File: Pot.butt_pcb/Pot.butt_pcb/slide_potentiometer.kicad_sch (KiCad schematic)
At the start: 16 parts

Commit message: main_func pcb done
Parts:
- RV13, RV14, RV15, RV16, RV17, RV18, RV19, RV20: footprint (none) -> Connector_PinSocket_2.54mm:PinSocket_1x03_P2.54mm_Horizontal
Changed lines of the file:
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@@
       (effects (font (size 1.27 1.27)) (justify right))
     )
-    (property "Footprint" "" (id 2) (at 243.84 46.99 0)
+    (property "Footprint" "Connector_PinSocket_2.54mm:PinSocket_1x03_P2.54mm_Horizontal" (id 2) (at 243.84 46.99 0)
       (effects (font (size 1.27 1.27)) hide)
     )
@@
       (effects (font (size 1.27 1.27)) (justify right))
     )
-    (property "Footprint" "" (id 2) (at 179.07 48.26 0)
+    (property "Footprint" "Connector_PinSocket_2.54mm:PinSocket_1x03_P2.54mm_Horizontal" (id 2) (at 179.07 48.26 0)
       (effects (font (size 1.27 1.27)) hide)
     )
@@
       (effects (font (size 1.27 1.27)) (justify right))
     )
-    (property "Footprint" "" (id 2) (at 52.07 44.45 0)
+    (property "Footprint" "Connector_PinSocket_2.54mm:PinSocket_1x03_P2.54mm_Horizontal" (id 2) (at 52.07 44.45 0)
       (effects (font (size 1.27 1.27)) hide)
     )
@@
       (effects (font (size 1.27 1.27)) (justify right))
     )
-    (property "Footprint" "" (id 2) (at 242.57 93.98 0)
+    (property "Footprint" "Connector_PinSocket_2.54mm:PinSocket_1x03_P2.54mm_Horizontal" (id 2) (at 242.57 93.98 0)
       (effects (font (size 1.27 1.27)) hide)
     )
@@
       (effects (font (size 1.27 1.27)) (justify right))
     )
-    (property "Footprint" "" (id 2) (at 179.07 93.98 0)
+    (property "Footprint" "Connector_PinSocket_2.54mm:PinSocket_1x03_P2.54mm_Horizontal" (id 2) (at 179.07 93.98 0)
       (effects (font (size 1.27 1.27)) hide)
     )
@@
       (effects (font (size 1.27 1.27)) (justify right))
     )
-    (property "Footprint" "" (id 2) (at 115.57 45.72 0)
+    (property "Footprint" "Connector_PinSocket_2.54mm:PinSocket_1x03_P2.54mm_Horizontal" (id 2) (at 115.57 45.72 0)
       (effects (font (size 1.27 1.27)) hide)
     )
@@
       (effects (font (size 1.27 1.27)) (justify right))
     )
-    (property "Footprint" "" (id 2) (at 115.57 93.98 0)
+    (property "Footprint" "Connector_PinSocket_2.54mm:PinSocket_1x03_P2.54mm_Horizontal" (id 2) (at 115.57 93.98 0)
       (effects (font (size 1.27 1.27)) hide)
     )
@@
       (effects (font (size 1.27 1.27)) (justify right))
     )
-    (property "Footprint" "" (id 2) (at 52.07 93.98 0)
-      (effects (font (size 1.27 1.27)) hide)
-    )
+    (property "Footprint" "Connector_PinSocket_2.54mm:PinSocket_1x03_P2.54mm_Horizontal" (id 2) (at 52.07 93.98 0)
+      (effects (font (size 1.27 1.27)) hide)
+    )

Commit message: Pot.but_pcb in progress
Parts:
- RV13, RV14, RV15, RV16, RV17, RV18, RV19, RV20: footprint Connector_PinSocket_2.54mm:PinSocket_1x03_P2.54mm_Horizontal -> Connector_PinSocket_2.54mm:PinSocket_1x03_P2.54mm_Vertical
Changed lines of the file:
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@@
       (effects (font (size 1.27 1.27)) (justify right))
     )
-    (property "Footprint" "Connector_PinSocket_2.54mm:PinSocket_1x03_P2.54mm_Horizontal" (id 2) (at 243.84 46.99 0)
+    (property "Footprint" "Connector_PinSocket_2.54mm:PinSocket_1x03_P2.54mm_Vertical" (id 2) (at 243.84 46.99 0)
       (effects (font (size 1.27 1.27)) hide)
     )
@@
       (effects (font (size 1.27 1.27)) (justify right))
     )
-    (property "Footprint" "Connector_PinSocket_2.54mm:PinSocket_1x03_P2.54mm_Horizontal" (id 2) (at 179.07 48.26 0)
+    (property "Footprint" "Connector_PinSocket_2.54mm:PinSocket_1x03_P2.54mm_Vertical" (id 2) (at 179.07 48.26 0)
       (effects (font (size 1.27 1.27)) hide)
     )
@@
       (effects (font (size 1.27 1.27)) (justify right))
     )
-    (property "Footprint" "Connector_PinSocket_2.54mm:PinSocket_1x03_P2.54mm_Horizontal" (id 2) (at 52.07 44.45 0)
+    (property "Footprint" "Connector_PinSocket_2.54mm:PinSocket_1x03_P2.54mm_Vertical" (id 2) (at 52.07 44.45 0)
       (effects (font (size 1.27 1.27)) hide)
     )
@@
       (effects (font (size 1.27 1.27)) (justify right))
     )
-    (property "Footprint" "Connector_PinSocket_2.54mm:PinSocket_1x03_P2.54mm_Horizontal" (id 2) (at 242.57 93.98 0)
+    (property "Footprint" "Connector_PinSocket_2.54mm:PinSocket_1x03_P2.54mm_Vertical" (id 2) (at 242.57 93.98 0)
       (effects (font (size 1.27 1.27)) hide)
     )
@@
       (effects (font (size 1.27 1.27)) (justify right))
     )
-    (property "Footprint" "Connector_PinSocket_2.54mm:PinSocket_1x03_P2.54mm_Horizontal" (id 2) (at 179.07 93.98 0)
+    (property "Footprint" "Connector_PinSocket_2.54mm:PinSocket_1x03_P2.54mm_Vertical" (id 2) (at 179.07 93.98 0)
       (effects (font (size 1.27 1.27)) hide)
     )
@@
       (effects (font (size 1.27 1.27)) (justify right))
     )
-    (property "Footprint" "Connector_PinSocket_2.54mm:PinSocket_1x03_P2.54mm_Horizontal" (id 2) (at 115.57 45.72 0)
+    (property "Footprint" "Connector_PinSocket_2.54mm:PinSocket_1x03_P2.54mm_Vertical" (id 2) (at 115.57 45.72 0)
       (effects (font (size 1.27 1.27)) hide)
     )
@@
       (effects (font (size 1.27 1.27)) (justify right))
     )
-    (property "Footprint" "Connector_PinSocket_2.54mm:PinSocket_1x03_P2.54mm_Horizontal" (id 2) (at 115.57 93.98 0)
+    (property "Footprint" "Connector_PinSocket_2.54mm:PinSocket_1x03_P2.54mm_Vertical" (id 2) (at 115.57 93.98 0)
       (effects (font (size 1.27 1.27)) hide)
     )
@@
       (effects (font (size 1.27 1.27)) (justify right))
     )
-    (property "Footprint" "Connector_PinSocket_2.54mm:PinSocket_1x03_P2.54mm_Horizontal" (id 2) (at 52.07 93.98 0)
-      (effects (font (size 1.27 1.27)) hide)
-    )
+    (property "Footprint" "Connector_PinSocket_2.54mm:PinSocket_1x03_P2.54mm_Vertical" (id 2) (at 52.07 93.98 0)
+      (effects (font (size 1.27 1.27)) hide)
+    )

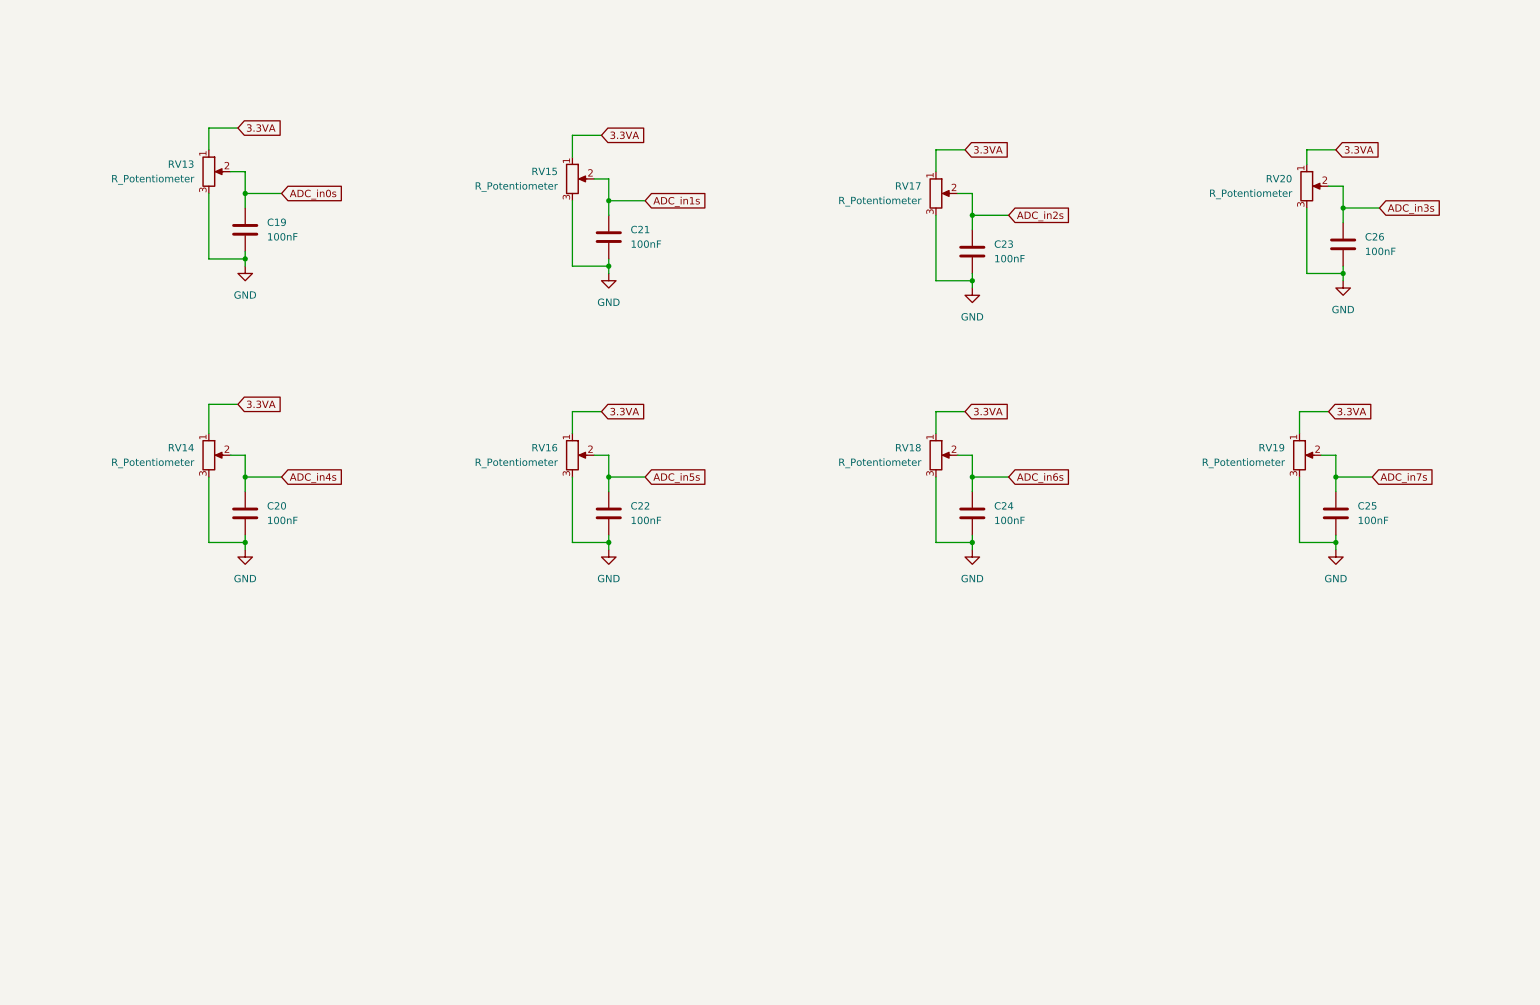
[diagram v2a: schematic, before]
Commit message: pcb design fixing
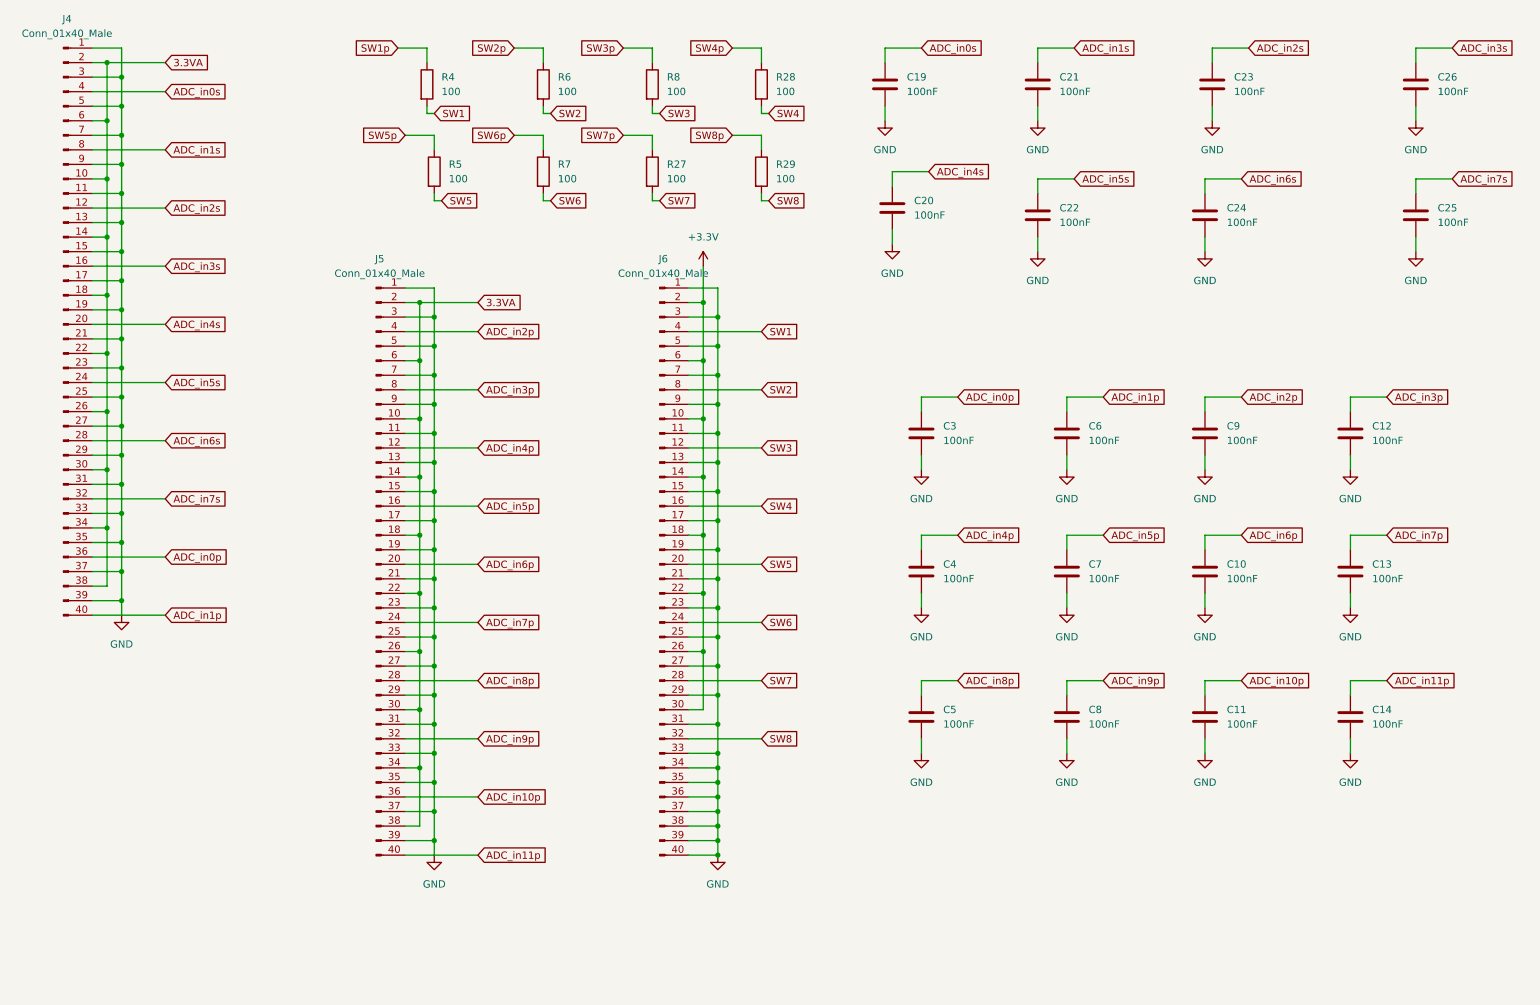
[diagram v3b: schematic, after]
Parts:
- removed RV13, RV14, RV15, RV16, RV17, RV18, RV19, RV20: R_Potentiometer, Connector_PinSocket_2.54mm:PinSocket_1x03_P2.54mm_Vertical, symbol Device:R_Potentiometer
- added C10, C11, C12, C13, C14, C3, C4, C5, C6, C7, C8, C9: 100nF, Capacitor_SMD:C_0805_2012Metric_Pad1.18x1.45mm_HandSolder, symbol Device:C
- added J4, J5, J6: Conn_01x40_Male, Connector_IDC:IDC-Header_2x20_P2.54mm_Vertical, symbol Connector:Conn_01x40_Male
- added R27, R28, R29, R4, R5, R6, R7, R8: 100, Resistor_SMD:R_0805_2012Metric_Pad1.20x1.40mm_HandSolder, symbol Device:R
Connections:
- net 3.3VA: now also J4.10 (Pin_10), J4.14 (Pin_14), J4.18 (Pin_18), J4.2 (Pin_2), J4.22 (Pin_22), J4.26 (Pin_26), J4.30 (Pin_30), J4.34 (Pin_34), J4.38 (Pin_38), J4.6 (Pin_6), J5.10 (Pin_10), J5.14 (Pin_14), J5.18 (Pin_18), J5.2 (Pin_2), J5.22 (Pin_22), J5.26 (Pin_26), J5.30 (Pin_30), J5.34 (Pin_34), J5.38 (Pin_38), J5.6 (Pin_6)
- net ADC_in0s: now also J4.4 (Pin_4)
- net ADC_in1s: now also J4.8 (Pin_8)
- net ADC_in2s: now also J4.12 (Pin_12)
- net ADC_in3s: now also J4.16 (Pin_16)
- net ADC_in4s: now also J4.20 (Pin_20)
- net ADC_in5s: now also J4.24 (Pin_24)
- net ADC_in6s: now also J4.28 (Pin_28)
- net ADC_in7s: now also J4.32 (Pin_32)
- net GND: now also C10.2, C11.2, C12.2, C13.2, C14.2, C3.2, C4.2, C5.2, C6.2, C7.2, C8.2, C9.2, J4.1 (Pin_1), J4.11 (Pin_11), J4.13 (Pin_13), J4.15 (Pin_15), J4.17 (Pin_17), J4.19 (Pin_19), J4.21 (Pin_21), J4.23 (Pin_23), J4.25 (Pin_25), J4.27 (Pin_27), J4.29 (Pin_29), J4.3 (Pin_3), J4.31 (Pin_31), J4.33 (Pin_33), J4.35 (Pin_35), J4.37 (Pin_37), J4.39 (Pin_39), J4.5 (Pin_5), J4.7 (Pin_7), J4.9 (Pin_9), J5.1 (Pin_1), J5.11 (Pin_11), J5.13 (Pin_13), J5.15 (Pin_15), J5.17 (Pin_17), J5.19 (Pin_19), J5.21 (Pin_21), J5.23 (Pin_23), J5.25 (Pin_25), J5.27 (Pin_27), J5.29 (Pin_29), J5.3 (Pin_3), J5.31 (Pin_31), J5.33 (Pin_33), J5.35 (Pin_35), J5.37 (Pin_37), J5.39 (Pin_39), J5.5 (Pin_5), J5.7 (Pin_7), J5.9 (Pin_9), J6.1 (Pin_1), J6.11 (Pin_11), J6.13 (Pin_13), J6.15 (Pin_15), J6.17 (Pin_17), J6.19 (Pin_19), J6.21 (Pin_21), J6.23 (Pin_23), J6.25 (Pin_25), J6.27 (Pin_27), J6.29 (Pin_29), J6.3 (Pin_3), J6.31 (Pin_31), J6.33 (Pin_33), J6.34 (Pin_34), J6.35 (Pin_35), J6.36 (Pin_36), J6.37 (Pin_37), J6.38 (Pin_38), J6.39 (Pin_39), J6.40 (Pin_40), J6.5 (Pin_5), J6.7 (Pin_7), J6.9 (Pin_9)
- new net +3V3: J6.10 (Pin_10), J6.14 (Pin_14), J6.18 (Pin_18), J6.2 (Pin_2), J6.22 (Pin_22), J6.26 (Pin_26), J6.30 (Pin_30), J6.6 (Pin_6)
- new net ADC_in0p: C3.1, J4.36 (Pin_36)
- new net ADC_in10p: C11.1, J5.36 (Pin_36)
- new net ADC_in11p: C14.1, J5.40 (Pin_40)
- new net ADC_in1p: C6.1, J4.40 (Pin_40)
- new net ADC_in2p: C9.1, J5.4 (Pin_4)
- new net ADC_in3p: C12.1, J5.8 (Pin_8)
- new net ADC_in4p: C4.1, J5.12 (Pin_12)
- new net ADC_in5p: C7.1, J5.16 (Pin_16)
- new net ADC_in6p: C10.1, J5.20 (Pin_20)
- new net ADC_in7p: C13.1, J5.24 (Pin_24)
- new net ADC_in8p: C5.1, J5.28 (Pin_28)
- new net ADC_in9p: C8.1, J5.32 (Pin_32)
- new net SW1: J6.4 (Pin_4), R4.2
- new net SW1p: R4.1
- new net SW2: J6.8 (Pin_8), R6.2
- new net SW2p: R6.1
- new net SW3: J6.12 (Pin_12), R8.2
- new net SW3p: R8.1
- new net SW4: J6.16 (Pin_16), R28.2
- new net SW4p: R28.1
- new net SW5: J6.20 (Pin_20), R5.2
- new net SW5p: R5.1
- new net SW6: J6.24 (Pin_24), R7.2
- new net SW6p: R7.1
- new net SW7: J6.28 (Pin_28), R27.2
- new net SW7p: R27.1
- new net SW8: J6.32 (Pin_32), R29.2
- new net SW8p: R29.1
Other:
- moved on the sheet: C19, C20, C21, C22, C23, C24, C25, C26

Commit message: gerber files generated
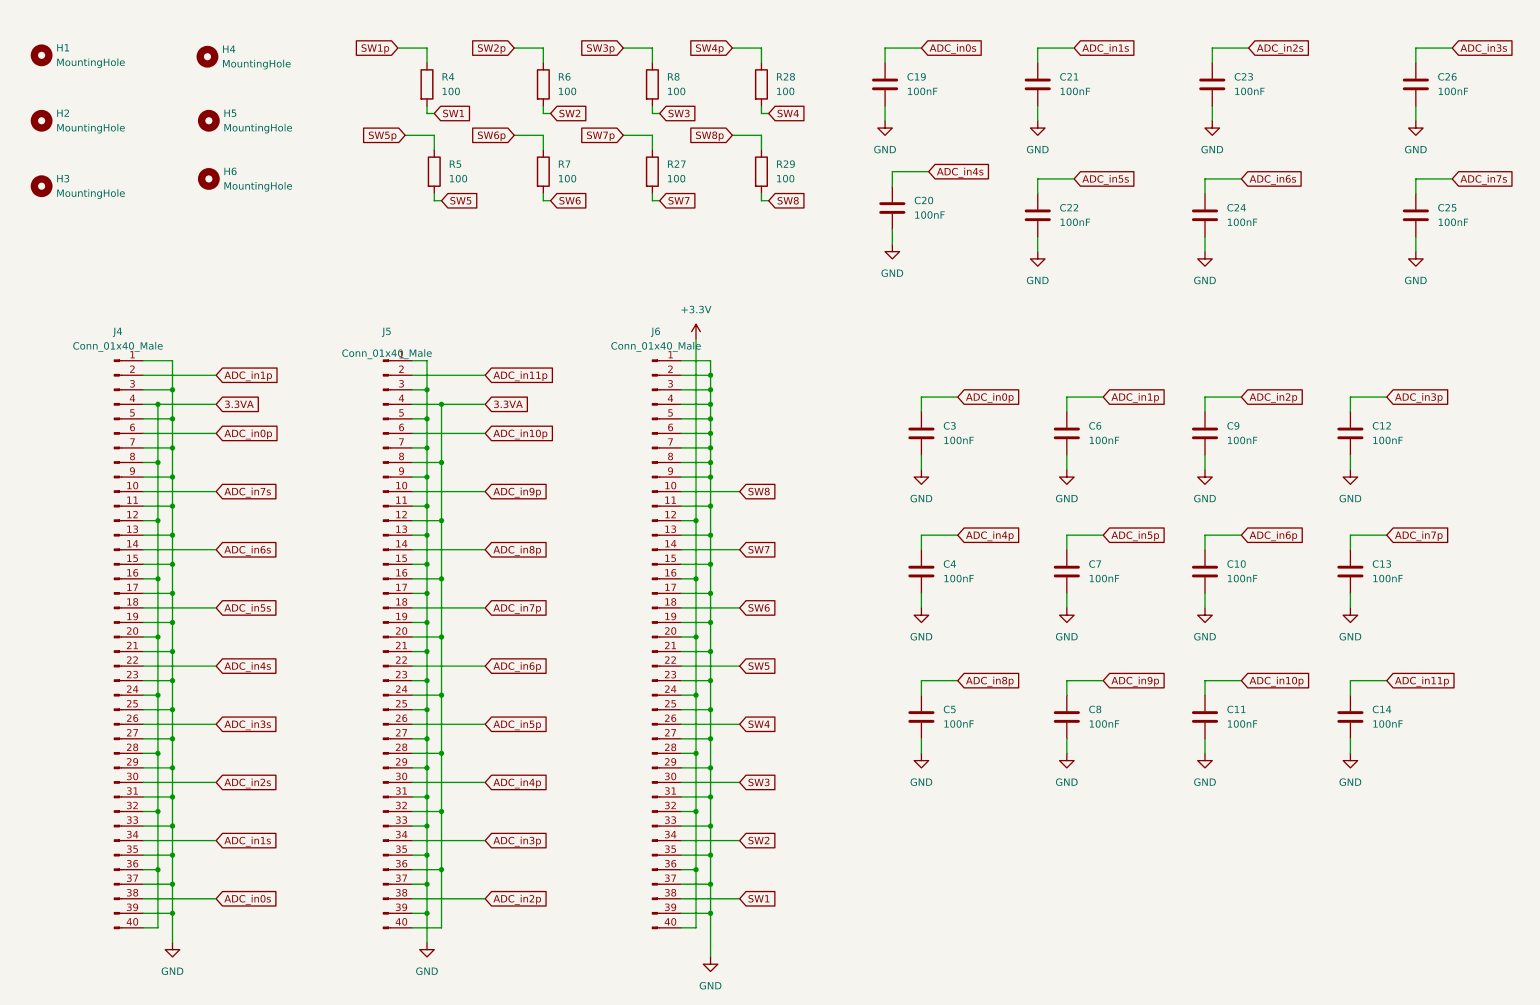
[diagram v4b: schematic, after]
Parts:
- added H1, H2, H3, H4, H5, H6: MountingHole, MountingHole:MountingHole_3.2mm_M3_Pad_Via, symbol Mechanical:MountingHole
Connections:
- net +3V3: now also J6.12 (Pin_12), J6.16 (Pin_16), J6.20 (Pin_20), J6.24 (Pin_24), J6.28 (Pin_28), J6.32 (Pin_32), J6.36 (Pin_36), J6.40 (Pin_40); no longer J6.10 (Pin_10), J6.14 (Pin_14), J6.18 (Pin_18), J6.2 (Pin_2), J6.22 (Pin_22), J6.26 (Pin_26), J6.30 (Pin_30), J6.6 (Pin_6)
- net 3.3VA: now also J4.12 (Pin_12), J4.16 (Pin_16), J4.20 (Pin_20), J4.24 (Pin_24), J4.28 (Pin_28), J4.32 (Pin_32), J4.36 (Pin_36), J4.4 (Pin_4), J4.40 (Pin_40), J4.8 (Pin_8), J5.12 (Pin_12), J5.16 (Pin_16), J5.20 (Pin_20), J5.24 (Pin_24), J5.28 (Pin_28), J5.32 (Pin_32), J5.36 (Pin_36), J5.4 (Pin_4), J5.40 (Pin_40), J5.8 (Pin_8); no longer J4.10 (Pin_10), J4.14 (Pin_14), J4.18 (Pin_18), J4.2 (Pin_2), J4.22 (Pin_22), J4.26 (Pin_26), J4.30 (Pin_30), J4.34 (Pin_34), J4.38 (Pin_38), J4.6 (Pin_6), J5.10 (Pin_10), J5.14 (Pin_14), J5.18 (Pin_18), J5.2 (Pin_2), J5.22 (Pin_22), J5.26 (Pin_26), J5.30 (Pin_30), J5.34 (Pin_34), J5.38 (Pin_38), J5.6 (Pin_6)
- net ADC_in0p: now also J4.6 (Pin_6); no longer J4.36 (Pin_36)
- net ADC_in0s: now also J4.38 (Pin_38); no longer J4.4 (Pin_4)
- net ADC_in10p: now also J5.6 (Pin_6); no longer J5.36 (Pin_36)
- net ADC_in11p: now also J5.2 (Pin_2); no longer J5.40 (Pin_40)
- net ADC_in1p: now also J4.2 (Pin_2); no longer J4.40 (Pin_40)
- net ADC_in1s: now also J4.34 (Pin_34); no longer J4.8 (Pin_8)
- net ADC_in2p: now also J5.38 (Pin_38); no longer J5.4 (Pin_4)
- net ADC_in2s: now also J4.30 (Pin_30); no longer J4.12 (Pin_12)
- net ADC_in3p: now also J5.34 (Pin_34); no longer J5.8 (Pin_8)
- net ADC_in3s: now also J4.26 (Pin_26); no longer J4.16 (Pin_16)
- net ADC_in4p: now also J5.30 (Pin_30); no longer J5.12 (Pin_12)
- net ADC_in4s: now also J4.22 (Pin_22); no longer J4.20 (Pin_20)
- net ADC_in5p: now also J5.26 (Pin_26); no longer J5.16 (Pin_16)
- net ADC_in5s: now also J4.18 (Pin_18); no longer J4.24 (Pin_24)
- net ADC_in6p: now also J5.22 (Pin_22); no longer J5.20 (Pin_20)
- net ADC_in6s: now also J4.14 (Pin_14); no longer J4.28 (Pin_28)
- net ADC_in7p: now also J5.18 (Pin_18); no longer J5.24 (Pin_24)
- net ADC_in7s: now also J4.10 (Pin_10); no longer J4.32 (Pin_32)
- net ADC_in8p: now also J5.14 (Pin_14); no longer J5.28 (Pin_28)
- net ADC_in9p: now also J5.10 (Pin_10); no longer J5.32 (Pin_32)
- net GND: now also J6.2 (Pin_2), J6.4 (Pin_4), J6.6 (Pin_6), J6.8 (Pin_8); no longer J6.34 (Pin_34), J6.36 (Pin_36), J6.38 (Pin_38), J6.40 (Pin_40)
- net SW1: now also J6.38 (Pin_38); no longer J6.4 (Pin_4)
- net SW2: now also J6.34 (Pin_34); no longer J6.8 (Pin_8)
- net SW3: now also J6.30 (Pin_30); no longer J6.12 (Pin_12)
- net SW4: now also J6.26 (Pin_26); no longer J6.16 (Pin_16)
- net SW5: now also J6.22 (Pin_22); no longer J6.20 (Pin_20)
- net SW6: now also J6.18 (Pin_18); no longer J6.24 (Pin_24)
- net SW7: now also J6.14 (Pin_14); no longer J6.28 (Pin_28)
- net SW8: now also J6.10 (Pin_10); no longer J6.32 (Pin_32)
